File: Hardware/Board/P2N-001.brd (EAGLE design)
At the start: 72 x 72 mm, 34 parts, among them IC1 4053N, IC2 LTC485N, IC3 74LS07N, IC4 LTC485N, K1 G5V1, T1 2SC1815

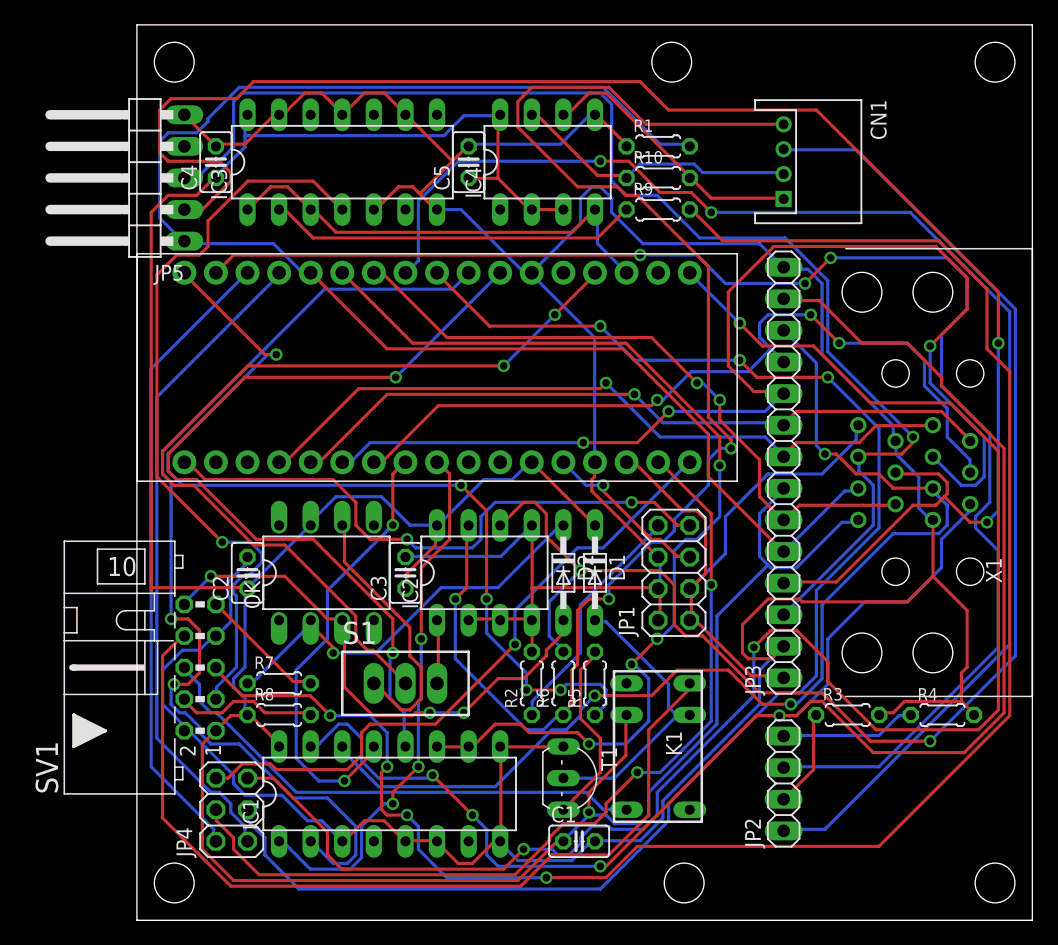
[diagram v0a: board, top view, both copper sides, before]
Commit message: Update document.
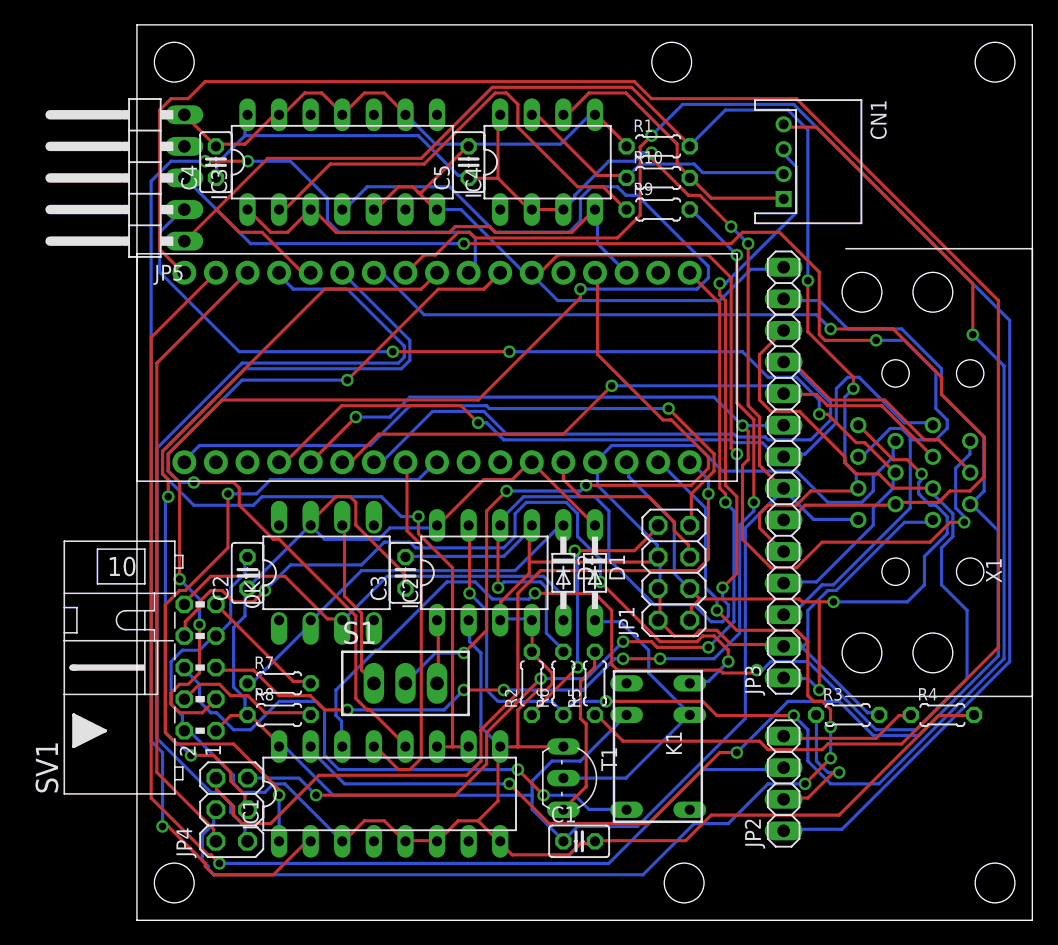
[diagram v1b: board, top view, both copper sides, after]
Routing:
- net N$22: track 75.4 -> 154.5 mm, vias 5 -> 0
- net N$10: track 143.2 -> 82.9 mm, vias 4 -> 7
- net N$9: track 120.3 -> 61.2 mm, vias 3 -> 2
- net N$11: track 133.1 -> 76.8 mm, vias 3 -> 5
- net N$1: track 61.1 -> 114.4 mm, vias 1 -> 3
- net N$25: track 135.3 -> 86.6 mm, vias 2 -> 3
- net ANLG2: track 95.3 -> 52.4 mm, vias 3 -> 1
- net N$29: track 142.8 -> 107.0 mm, vias 4 -> 2
- net GND: track 333.4 -> 368.5 mm, vias 0 -> 1
- net MIDI11: track 115.8 -> 83.3 mm, vias 2 -> 3
- net N$27: track 53.4 -> 76.1 mm, vias 2 -> 1
- net N$33: track 71.3 -> 92.4 mm, vias 2 -> 4
- net N$28: track 89.5 -> 110.3 mm, vias 3 -> 2
- net ANLG1: track 57.9 -> 78.3 mm, vias 1 -> 3
- net N$19: track 80.7 -> 100.5 mm, vias 2 -> 3
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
